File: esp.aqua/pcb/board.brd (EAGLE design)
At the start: 66.8 x 74.9 mm, 18 parts, among them Q1 BC849SMD, U1 XPT2046

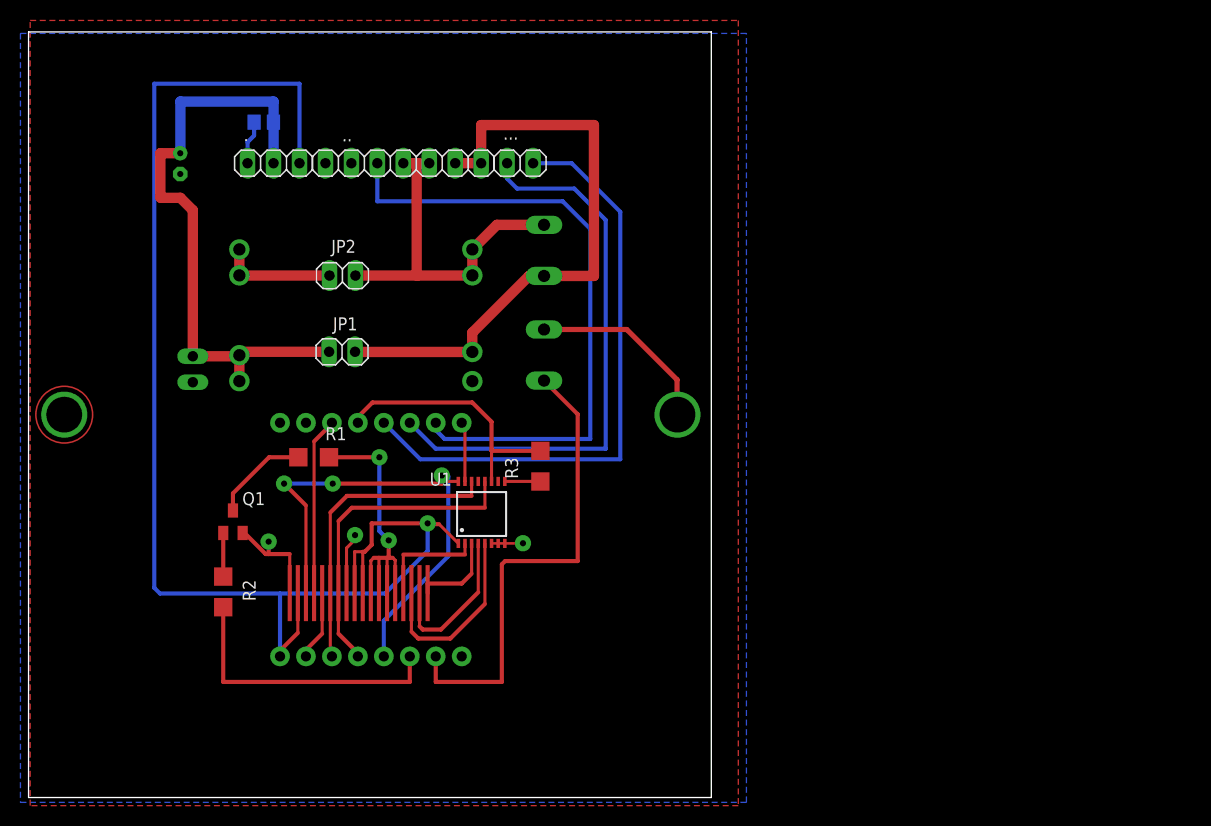
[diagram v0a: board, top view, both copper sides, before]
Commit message: first
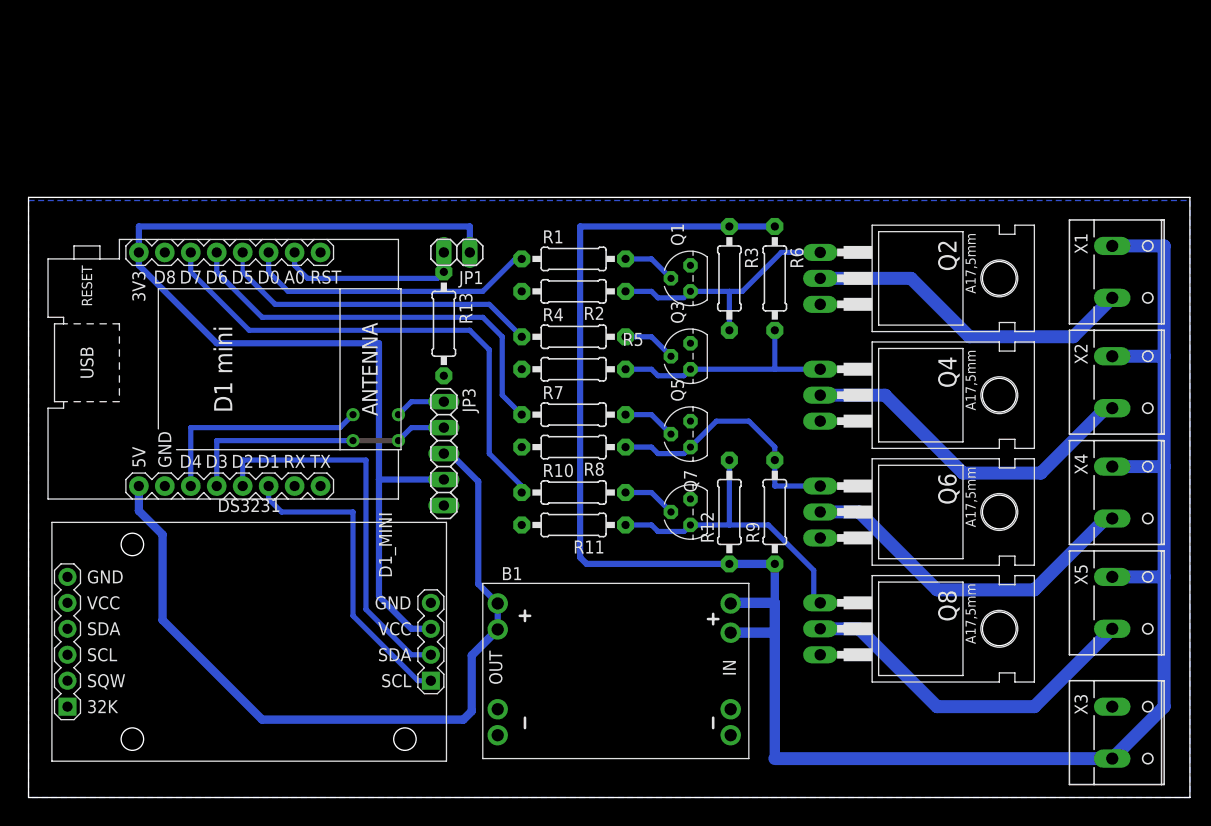
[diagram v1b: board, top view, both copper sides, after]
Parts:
- removed .: (no value), pinhead:1X03
- removed ..: (no value), pinhead:1X07
- removed ..., JP2, JP4: (no value), pinhead:1X02
- removed C1: (no value), rcl:C0805
- removed C3: (no value), rcl:E2-5
- removed U$2: 2.4TTF, eagle1:TFT2.4
- removed U1: XPT2046, eagle1:TSSOP16
- added DS3231: RTC-DS3231-AT24C32, diy-modules:RTC-DS3231-AT24C32
- added JP3: (no value), pinhead:1X05
- added Q2, Q4, Q6, Q8: IRF540, transistor-fet:TO220
- added Q3, Q5, Q7: BC547, transistor-npn:TO92
- added R10, R11, R12, R13, R4, R5, R6, R7, R8, R9: (no value), rcl:0207/10
- added X3, X4, X5: (no value), con-wago-508:W237-132
- Q1: value BC849SMD -> BC547; device transistor-npn:SOT23-BEC -> transistor-npn:TO92
- R1: value 2R5 -> (none); device rcl:R1210W -> rcl:0207/10
- R2, R3: value 1K -> (none); device rcl:R1210W -> rcl:0207/10
- X1, X2: device con-wago-500:W237-102 -> con-wago-508:W237-132
- moved X2 57.6 mm to (106.7, 40.6), flipped to the top
- moved X1 57.5 mm to (106.7, 51.4), flipped to the top
- moved Q1 50.7 mm to (64.8, 50.8), turned to 90 degrees
- moved B1 47.9 mm to (53.3, 9.53), flipped to the top, turned to 0 degrees
- moved R2 45.2 mm to (53.3, 49.5), turned to 180 degrees
- moved R1 32.0 mm to (53.3, 52.7), turned to 0 degrees
- moved R3 26.1 mm to (68.6, 50.8), turned to 270 degrees
- moved D1_MINI 21.6 mm to (19.1, 41.9), flipped to the top, turned to 270 degrees
- moved JP1 14.9 mm to (41.9, 53.3)
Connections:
- removed net DC: D1_MINI.JP2.6, U$2.P$4
- removed net IN-: ...3, ...4, B1.VIN-1, B1.VIN-2, JP2.1, X1.1
- removed net LED: D1_MINI.JP1.3, R2.2
- removed net LED+: ...6
- removed net LED-: ...7
- removed net MISO: D1_MINI.JP1.5, U$2.P$7, U1.12
- removed net MOSI: D1_MINI.JP1.6, U$2.P$6, U1.14
- removed net N$2: R1.1, U$2.P$11, U$2.P$12, U$2.P$13, U$2.P$14
- removed net OUT: ..2, B1.VOUT+1, B1.VOUT+2, C1.1, C3.+, JP1.2, JP4.1
- removed net SCK: D1_MINI.JP1.4, U$2.P$3, U1.16
- removed net T_IRQ: D1_MINI.JP2.5, R3.2, U1.11
- removed net VCC: D1_MINI.JP2.8, JP4.2
- removed net XN: U$2.P$17, U1.4
- removed net XP: U$2.P$15, U1.2
- removed net YN: U$2.P$16, U1.5
- removed net YP: U$2.P$18, U1.3
- new net 12: D1_MINI.JP1.5, R7.1
- new net 13: D1_MINI.JP1.6, R10.1
- new net 14: D1_MINI.JP1.4, R4.1
- new net 16: D1_MINI.JP1.3, R1.1
- new net 5V: B1.VOUT+1, B1.VOUT+2, D1_MINI.JP2.8, JP3.3
- new net D3: D1_MINI.JP2.5, JP3.2
- new net D4: D1_MINI.JP2.6, JP3.1
- new net N$1: Q1.2, R1.2
- new net N$11: Q5.3, Q6.1, R8.1, R9.2
- new net N$12: Q6.2, X4.2
- new net N$13: Q7.2, R10.2
- new net N$14: DS3231.J1.6
- new net N$15: DS3231.J1.5
- new net N$17: Q7.3, Q8.1, R11.1, R12.2
- new net N$18: Q8.2, X5.2
- new net N$7: Q3.3, Q4.1, R5.1, R6.2
- new net N$8: Q4.2, X2.2
- new net N$9: Q5.2, R7.2
- net 3V3: now also DS3231.J2.3, JP1.1, JP3.4; no longer ..3, U$2.P$10, U$2.P$2, U$2.P$9, U1.1
- net A0: now also JP1.2, R13.1; no longer X2.2
- net CS: no longer U$2.P$5
- net GND: now also B1.VIN-1, B1.VIN-2, DS3231.J2.4, JP3.5, Q1.1, Q2.3, Q3.1, Q4.3, Q5.1, Q6.3, Q7.1, Q8.3, R11.2, R13.2, R2.2, R5.2, R8.2, X3.1; no longer ..1, C1.2, C3.-, JP2.2, Q1.E, U$2.P$1, U$2.P$8, U1.6, U1.7, U1.8, X2.1
- net IN+: now also B1.EN, R12.1, R3.1, R6.1, R9.1, X1.1, X2.1, X3.2, X4.1, X5.1; no longer ...1, ...2, JP1.1, X1.2
- net N$3: now also Q1.3, Q2.1, R2.1, R3.2; no longer Q1.C, R1.2
- net N$4: now also Q3.2, R4.2; no longer Q1.B, R2.1
- net N$5: now also Q2.2, X1.2; no longer R3.1, U1.9
- net PWM: no longer ...5
- net SCL: now also DS3231.J2.1; no longer ....1
- net SDA: now also DS3231.J2.2; no longer ....2
- net TX: no longer U1.15
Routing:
- net IN+: track 60.1 -> 204.2 mm
- net 5V: track 0.00 -> 77.5 mm
- net PWM: track 62.4 -> 0.00 mm
- net OUT: track 60.5 -> 0.00 mm
- net GND: track 53.7 -> 0.00 mm, vias 5 -> 0
- net SCK: track 51.0 -> 0.00 mm, vias 3 -> 0
- net 13: track 0.00 -> 49.6 mm
- net 12: track 0.00 -> 40.9 mm
- net IN-: track 35.6 -> 0.00 mm
- net N$18: track 0.00 -> 34.9 mm
- net N$12: track 0.00 -> 34.6 mm
- net 3V3: track 137.3 -> 102.9 mm, vias 1 -> 0
- net N$8: track 0.00 -> 34.4 mm
- net 14: track 0.00 -> 31.8 mm
- net MISO: track 31.5 -> 0.00 mm
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- removed copper zone on layer 1, net VCC
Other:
- board size 66.8 x 74.9 mm -> 113.6 x 58.7 mm
- board text removed: "3v3"
- board text removed: "GND"
- board text removed: "IN+"
- board text removed: "IN-"
- board text removed: "LED+"
- board text removed: "LED-"
- board text removed: "PWM"
- board text removed: "SCL"
- board text removed: "SDA"
- board text removed: "SIG"
- board text removed: "VCC"
